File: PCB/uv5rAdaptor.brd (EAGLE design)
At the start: 13.9 x 13.9 mm, 2 parts

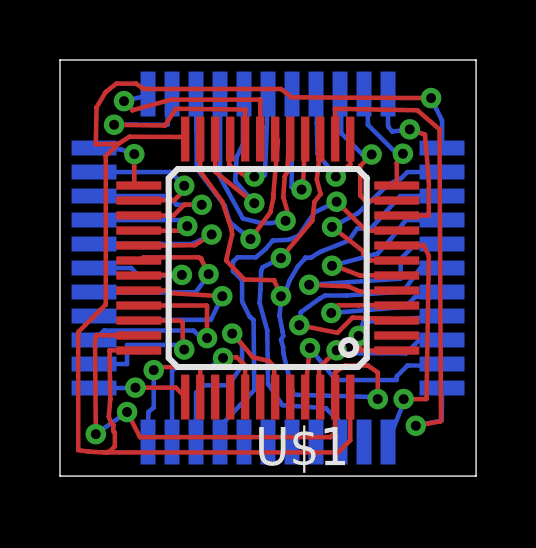
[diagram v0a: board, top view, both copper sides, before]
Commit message: Cleanup Routes
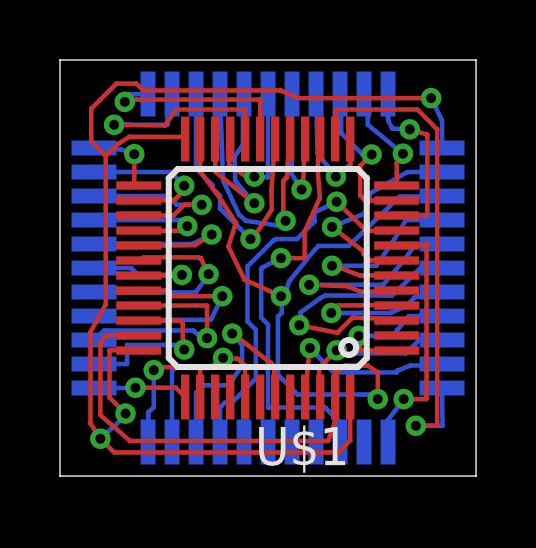
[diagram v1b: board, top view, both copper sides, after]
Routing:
- net VSS: track 38.1 -> 36.7 mm, vias 4 -> 2
- net VDD: track 43.9 -> 42.6 mm, vias 1 -> 3
- net TONE: track 12.7 -> 13.6 mm
- net AVDD: track 13.5 -> 13.0 mm
